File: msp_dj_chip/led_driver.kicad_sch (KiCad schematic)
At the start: 26 parts, among them J23 Conn_01x10_Socket, J24 Conn_01x10_Socket, U17 SSM6N7002KFU, U18 SSM6N7002KFU, U19 SSM6N7002KFU, U20 SSM6N7002KFU, U21 SSM6N7002KFU, U22 SSM6N7002KFU, U23 SSM6N7002KFU, U24 SSM6N7002KFU

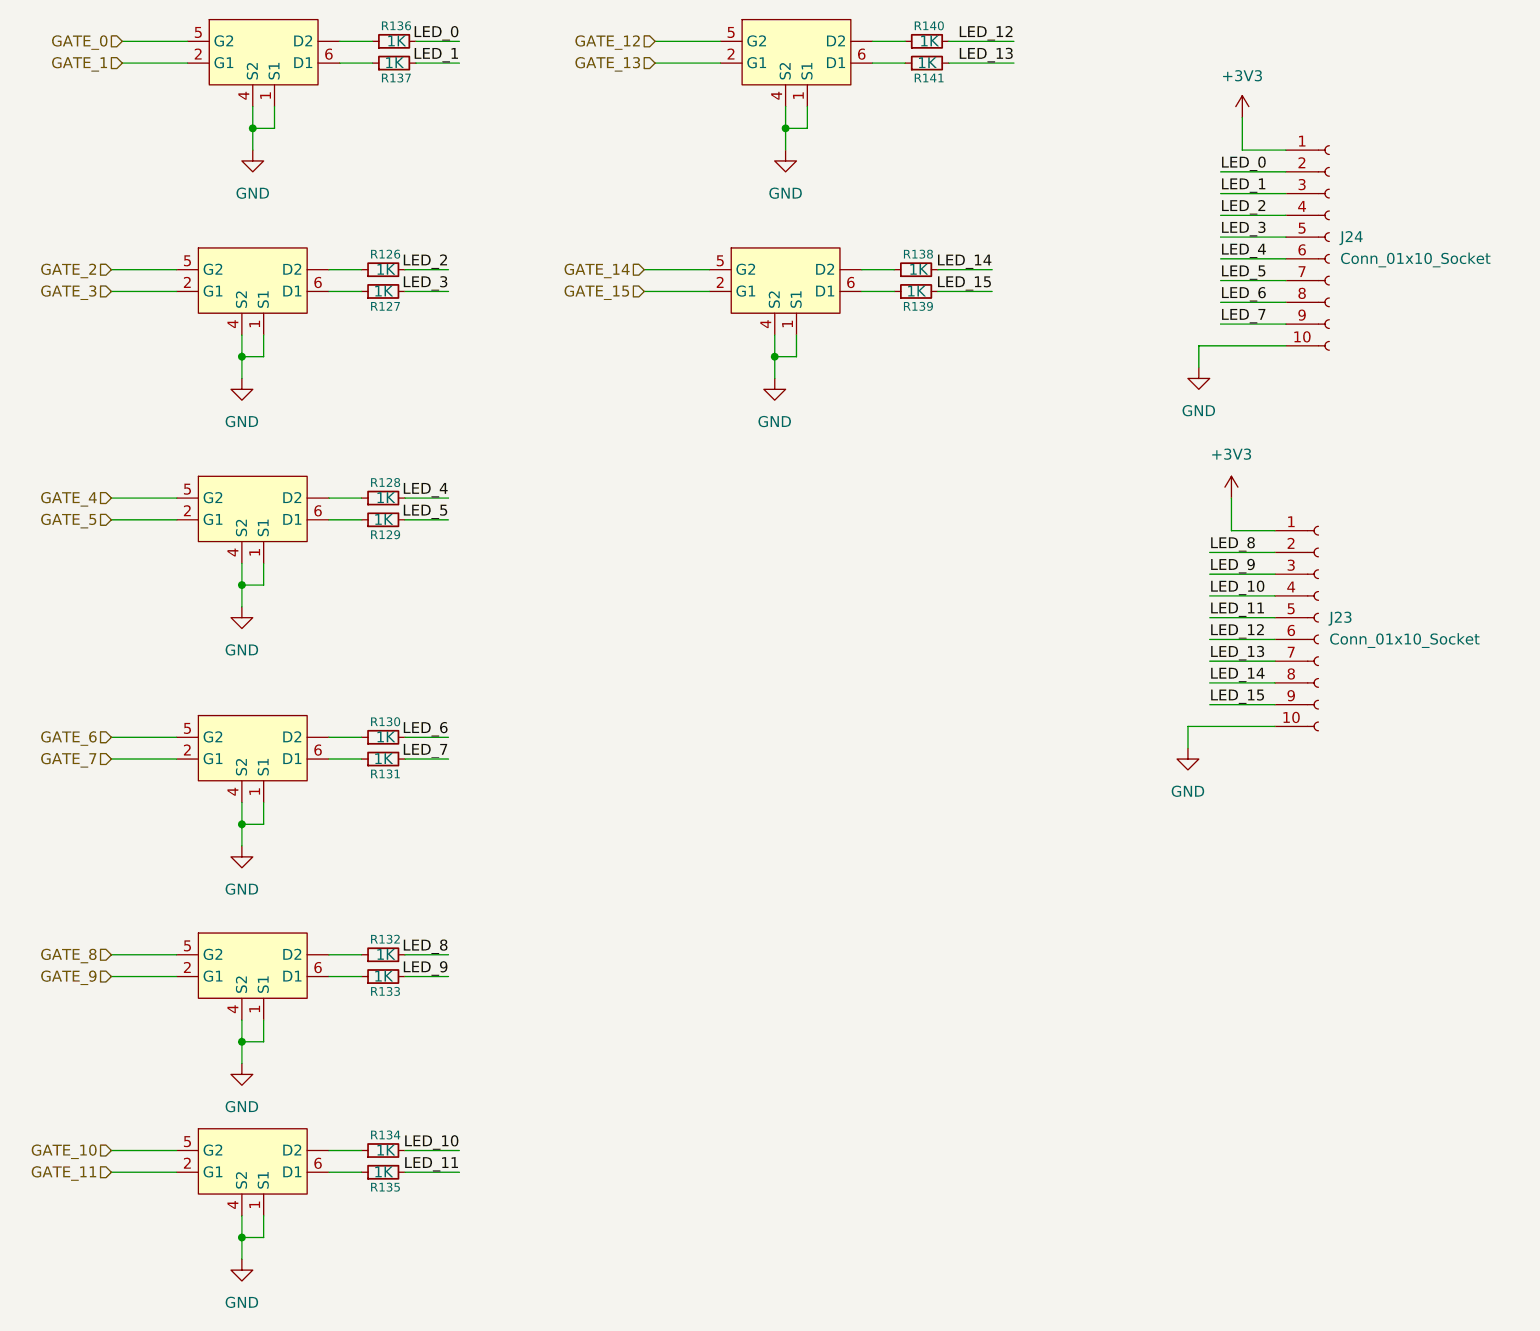
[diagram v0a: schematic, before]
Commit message: mark changes
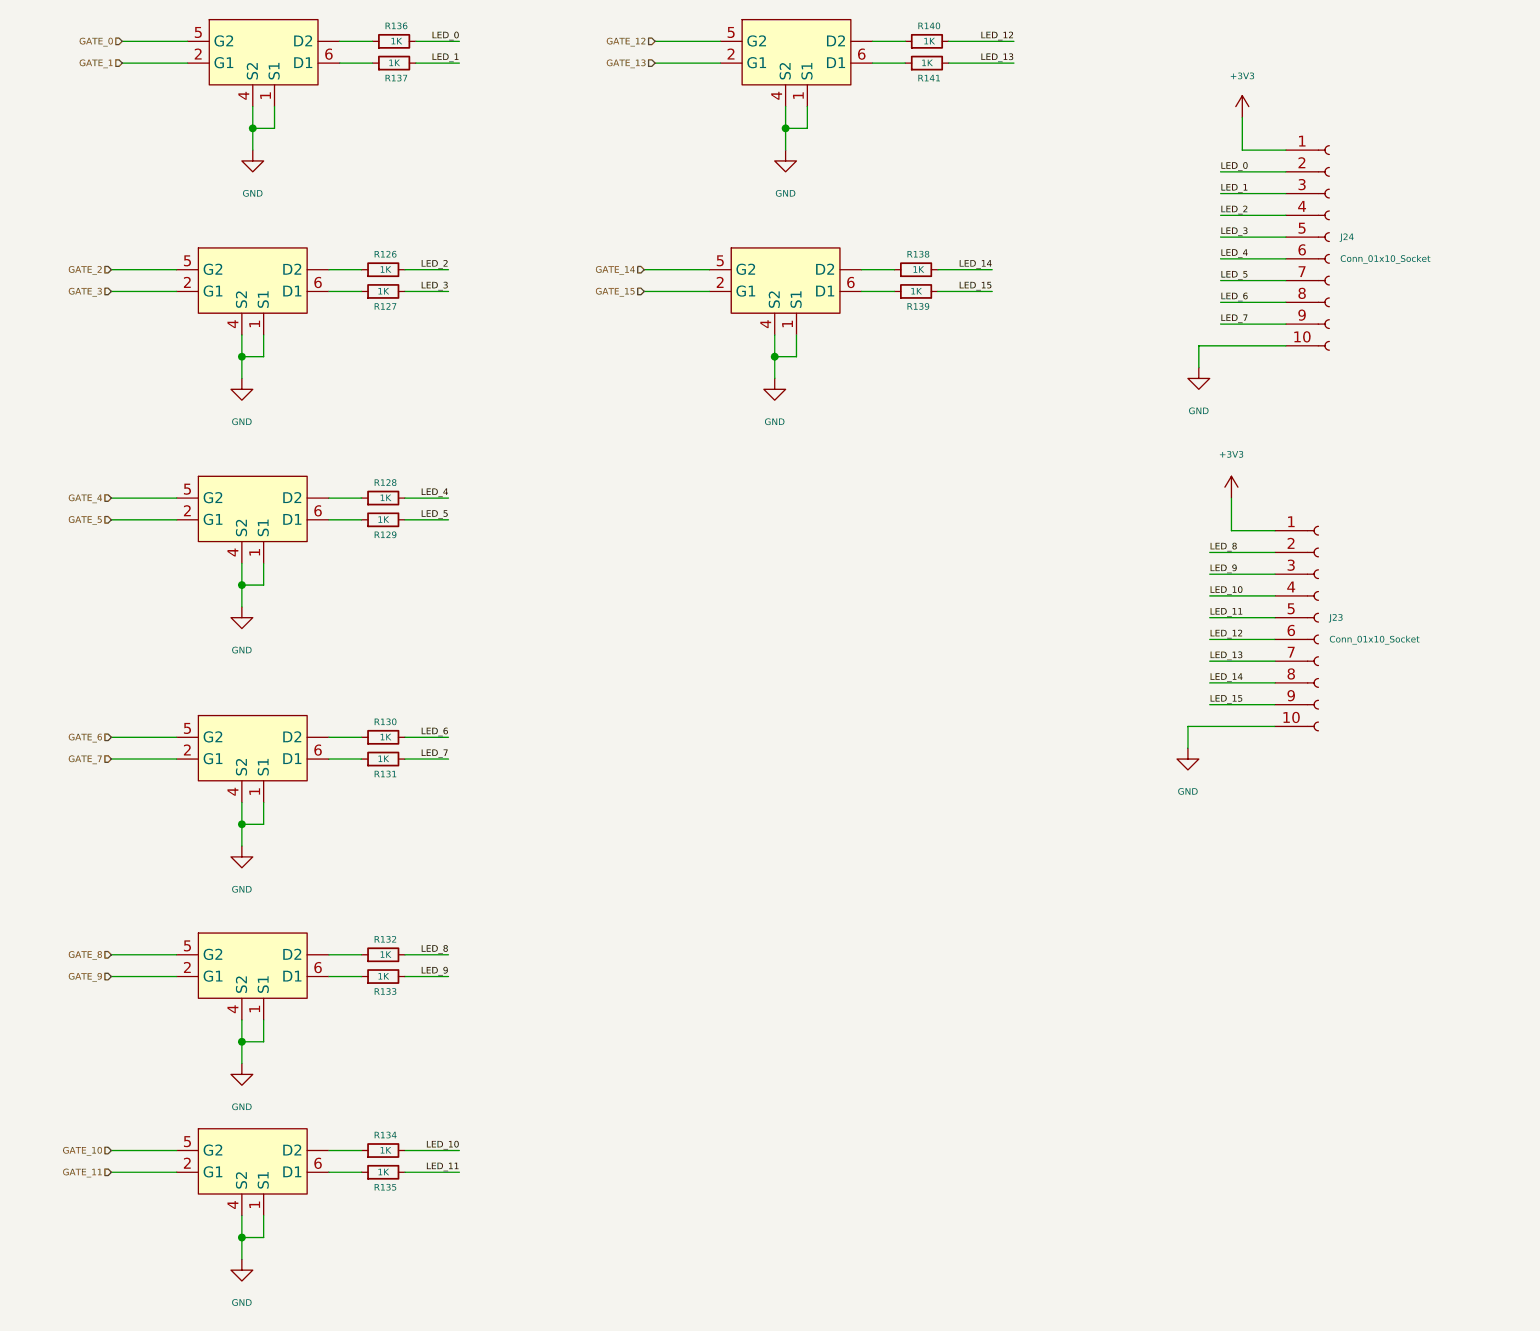
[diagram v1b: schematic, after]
